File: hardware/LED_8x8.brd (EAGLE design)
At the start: 86 x 82.5 mm, 13 parts, among them IC1 74HC595N, Q1 BC548, Q2 BC548, Q3 BC548, Q4 BC548, Q5 BC548, Q6 BC548, Q7 BC548, Q8 BC548

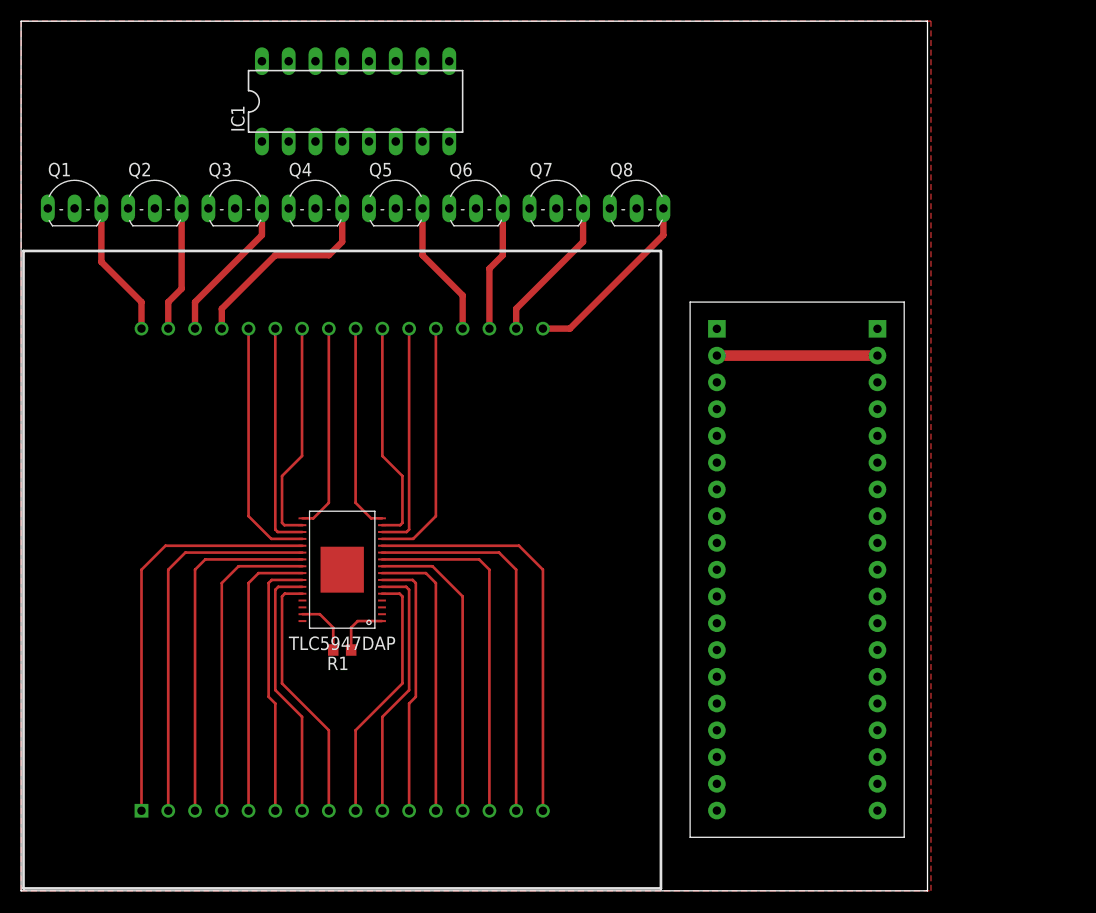
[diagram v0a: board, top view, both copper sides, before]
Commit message: finished layout
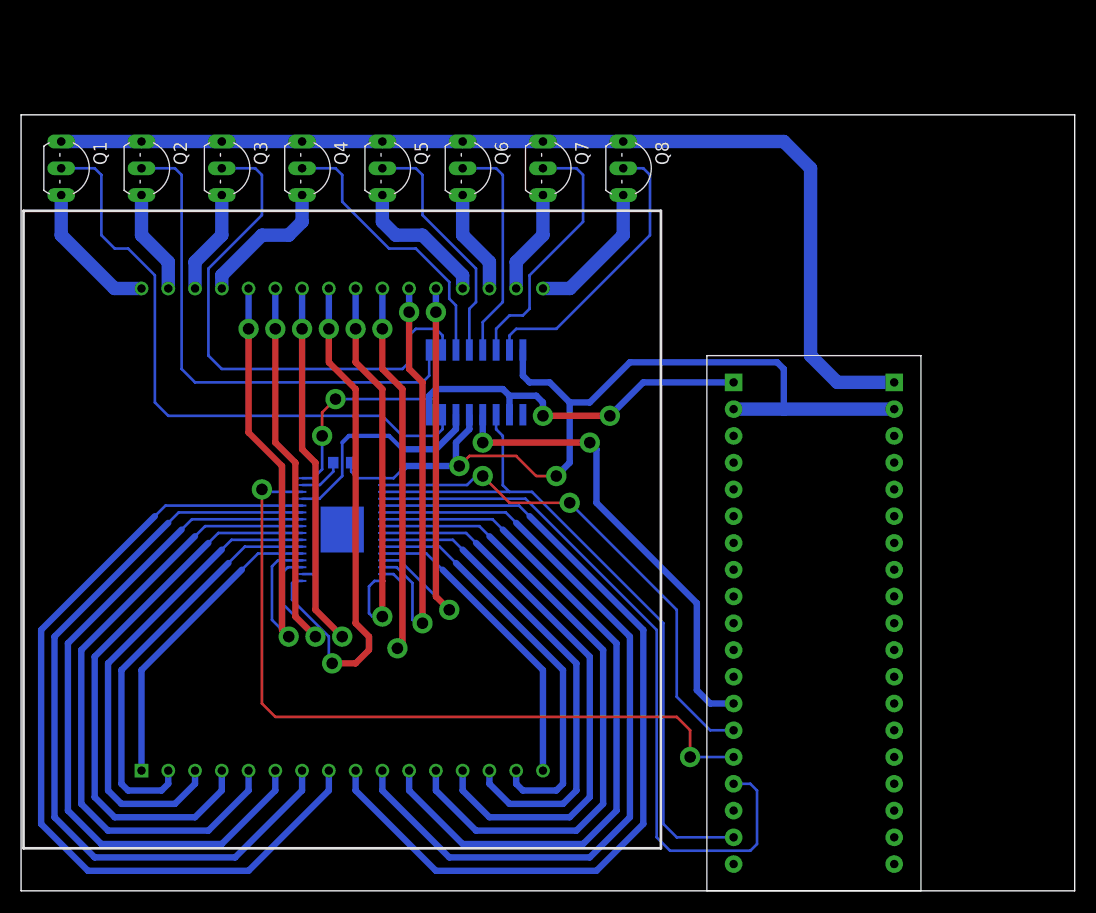
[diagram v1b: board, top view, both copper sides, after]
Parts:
- IC1: value 74HC595N -> 74HC595D; device 74xx-eu:DIL16 -> 74xx-eu:SO16
- moved IC1 29.0 mm to (43.2, 48.3), flipped to the bottom, turned to 180 degrees
- moved R1 17.8 mm to (30.5, 40.6), flipped to the bottom, turned to 0 degrees
- moved U$2 5.32 mm to (75.2, 25.4)
- moved U$1 3.81 mm to (30.5, 34.3), flipped to the bottom, turned to 0 degrees
- moved U$3 3.81 mm to (30.5, 34.3)
- moved Q1 2.54 mm to (5.08, 68.6), turned to 270 degrees
- moved Q2 2.54 mm to (12.7, 68.6), turned to 270 degrees
- moved Q3 2.54 mm to (20.3, 68.6), turned to 270 degrees
- moved Q4 2.54 mm to (27.9, 68.6), turned to 270 degrees
- moved Q5 2.54 mm to (35.6, 68.6), turned to 270 degrees
- moved Q6 2.54 mm to (43.2, 68.6), turned to 270 degrees
- moved Q7 2.54 mm to (50.8, 68.6), turned to 270 degrees
- moved Q8 2.54 mm to (58.4, 68.6), turned to 270 degrees
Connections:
- removed net VDD: U$2.VUSB
- new net +5V: Q1.C, Q2.C, Q3.C, Q4.C, Q5.C, Q6.C, Q7.C, Q8.C, U$2.VUSB
- net VCC: no longer Q1.C, Q2.C, Q3.C, Q4.C, Q5.C, Q6.C, Q7.C, Q8.C
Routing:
- net +5V: track 0.00 -> 98.9 mm
- net XLAT: track 0.00 -> 72.6 mm, vias 0 -> 2
- net MOSI: track 0.00 -> 68.8 mm
- net SCK: track 0.00 -> 66.0 mm
- net GND: track 20.5 -> 84.9 mm, vias 0 -> 2
- net SHIFTA1: track 0.00 -> 58.8 mm
- net RED1: track 24.2 -> 82.3 mm
- net BLUE8: track 24.2 -> 82.3 mm
- net VCC: track 0.00 -> 54.2 mm, vias 0 -> 4
- net SHIFTA3: track 0.00 -> 50.8 mm
- net RED2: track 24.7 -> 75.1 mm
- net BLUE7: track 24.7 -> 75.1 mm
- net SHIFTA2: track 0.00 -> 49.2 mm
- net BLANK: track 0.00 -> 48.6 mm, vias 0 -> 2
- net RCK: track 0.00 -> 44.5 mm, vias 0 -> 2
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- removed copper zone on layer 1, net N$2
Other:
- board size 86 x 82.5 mm -> 100 x 73.7 mm
